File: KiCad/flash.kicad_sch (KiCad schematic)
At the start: 3 parts, among them IC4 W25Q32JWSNIQ

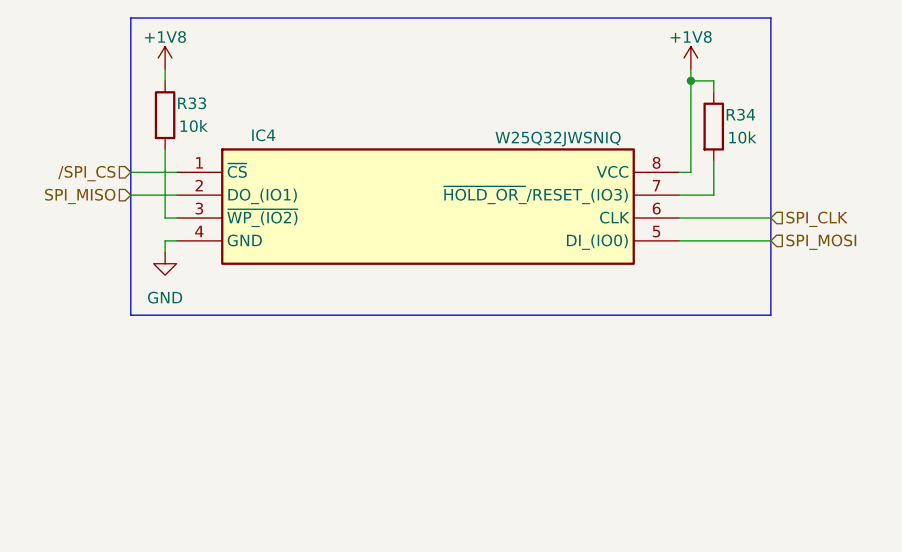
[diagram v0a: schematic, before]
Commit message: Added some TODOs, fixed some TODOs
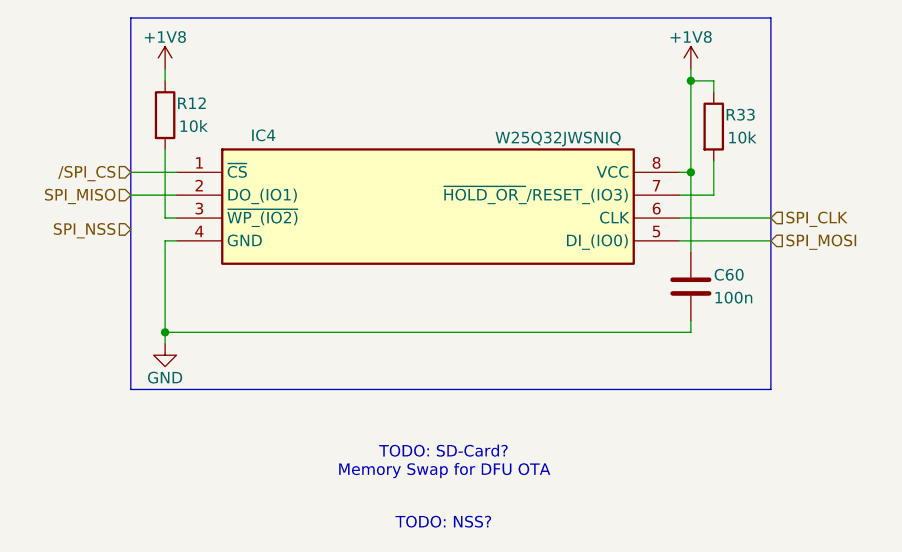
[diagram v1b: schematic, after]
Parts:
- added C60: 100n, Capacitor_SMD:C_0402_1005Metric, symbol Device:C
- renumbered R33 to R12, R34 to R33
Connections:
- net +1V8: now also C60.1
- net GND: now also C60.2
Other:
- note added: "TODO: NSS?"
- note added: "TODO: SD-Card? Memory Swap for DFU OTA"
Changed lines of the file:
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@@
 	(rectangle
 		(start 132.08 37.465)
-		(end 203.2 70.485)
+		(end 203.2 78.74)
 		(stroke
 			(width 0)
@@
 		(fill
 			(type none)
+		)
+	)
+	(text "TODO: NSS?"
+		(exclude_from_sim no)
+		(at 166.878 93.726 0)
+		(effects
+			(font
+				(size 1.27 1.27)
+			)
+		)
+	)
+	(text "TODO: SD-Card?\nMemory Swap for DFU OTA"
+		(exclude_from_sim no)
+		(at 166.878 86.868 0)
+		(effects
+			(font
+				(size 1.27 1.27)
+			)
 		)
 	)
@@
 		(color 0 0 0 0)
 	)
+	(junction
+		(at 135.89 72.39)
+		(diameter 0)
+		(color 0 0 0 0)
+	)
+	(junction
+		(at 194.31 54.61)
+		(diameter 0)
+		(color 0 0 0 0)
+	)
 	(wire
 		(pts
@@
 	(wire
 		(pts
+			(xy 135.89 73.66) (xy 135.89 72.39)
+		)
+		(stroke
+			(width 0)
+			(type default)
+		)
+	)
+	(wire
+		(pts
 			(xy 196.85 44.45) (xy 194.31 44.45)
 		)
@@
 	(wire
 		(pts
-			(xy 135.89 62.23) (xy 135.89 63.5)
-		)
-		(stroke
-			(width 0)
-			(type default)
-		)
-	)
-	(wire
-		(pts
 			(xy 135.89 43.18) (xy 135.89 44.45)
 		)
@@
 	(wire
 		(pts
+			(xy 194.31 72.39) (xy 194.31 71.12)
+		)
+		(stroke
+			(width 0)
+			(type default)
+		)
+	)
+	(wire
+		(pts
+			(xy 135.89 72.39) (xy 194.31 72.39)
+		)
+		(stroke
+			(width 0)
+			(type default)
+		)
+	)
+	(wire
+		(pts
 			(xy 137.16 59.69) (xy 135.89 59.69)
 		)
@@
 		(pts
 			(xy 132.08 54.61) (xy 137.16 54.61)
+		)
+		(stroke
+			(width 0)
+			(type default)
+		)
+	)
+	(wire
+		(pts
+			(xy 135.89 62.23) (xy 135.89 72.39)
+		)
+		(stroke
+			(width 0)
+			(type default)
+		)
+	)
+	(wire
+		(pts
+			(xy 194.31 54.61) (xy 194.31 63.5)
 		)
 		(stroke
@@
 		)
 	)
+	(hierarchical_label "SPI_NSS"
+		(shape input)
+		(at 132.08 60.96 180)
+		(effects
+			(font
+				(size 1.27 1.27)
+			)
+			(justify right)
+		)
+	)
 	(hierarchical_label "SPI_MOSI"
 		(shape input)
@@
 	(symbol
 		(lib_id "power:GND")
-		(at 135.89 63.5 0)
+		(at 135.89 73.66 0)
 		(unit 1)
 		(exclude_from_sim no)
@@
 		(on_board yes)
 		(dnp no)
-		(fields_autoplaced yes)
-		(property "Reference" "#PWR050"
-			(at 135.89 69.85 0)
+		(property "Reference" "#PWR048"
+			(at 135.89 80.01 0)
 			(effects
 				(font
@@
 		)
 		(property "Value" "GND"
-			(at 135.89 68.58 0)
+			(at 135.89 77.47 0)
 			(effects
 				(font
@@
 		)
 		(property "Footprint" ""
-			(at 135.89 63.5 0)
+			(at 135.89 73.66 0)
 			(effects
 				(font
@@
 		)
 		(property "Datasheet" ""
-			(at 135.89 63.5 0)
+			(at 135.89 73.66 0)
 			(effects
 				(font
@@
 		)
 		(property "Description" "Power symbol creates a global label with name \"GND\" , ground"
-			(at 135.89 63.5 0)
+			(at 135.89 73.66 0)
 			(effects
 				(font
@@
 		)
 		(instances
-			(project ""
-				(path "/643c756f-a801-466b-9148-7370ee6a5e00/75654986-1960-401a-97fe-a40bfa802dfa"
-					(reference "#PWR050")
+			(project "STDC"
+				(path "/643c756f-a801-466b-9148-7370ee6a5e00/a5768ca1-322e-4c77-bc87-c3070b355a8f"
+					(reference "#PWR048")
 					(unit 1)
 				)
@@
 		(on_board yes)
 		(dnp no)
-		(property "Reference" "#PWR049"
+		(property "Reference" "#PWR021"
 			(at 194.31 46.99 0)
 			(effects
@@
 		)
 		(instances
-			(project ""
-				(path "/643c756f-a801-466b-9148-7370ee6a5e00/75654986-1960-401a-97fe-a40bfa802dfa"
-					(reference "#PWR049")
+			(project "STDC"
+				(path "/643c756f-a801-466b-9148-7370ee6a5e00/a5768ca1-322e-4c77-bc87-c3070b355a8f"
+					(reference "#PWR021")
 					(unit 1)
 				)
@@
 		(on_board yes)
 		(dnp no)
-		(property "Reference" "R34"
+		(property "Reference" "R33"
 			(at 198.12 48.26 0)
 			(effects
@@
 		(instances
 			(project "STDC"
-				(path "/643c756f-a801-466b-9148-7370ee6a5e00/75654986-1960-401a-97fe-a40bfa802dfa"
-					(reference "R34")
+				(path "/643c756f-a801-466b-9148-7370ee6a5e00/a5768ca1-322e-4c77-bc87-c3070b355a8f"
+					(reference "R33")
 					(unit 1)
 				)
@@
 		(on_board yes)
 		(dnp no)
-		(property "Reference" "R33"
+		(property "Reference" "R12"
 			(at 137.16 46.99 0)
 			(effects
@@
 		)
 		(instances
-			(project ""
-				(path "/643c756f-a801-466b-9148-7370ee6a5e00/75654986-1960-401a-97fe-a40bfa802dfa"
-					(reference "R33")
+			(project "STDC"
+				(path "/643c756f-a801-466b-9148-7370ee6a5e00/a5768ca1-322e-4c77-bc87-c3070b355a8f"
+					(reference "R12")
+					(unit 1)
+				)
+			)
+		)
+	)
+	(symbol
+		(lib_id "Device:C")
+		(at 194.31 67.31 0)
+		(unit 1)
+		(exclude_from_sim no)
+		(in_bom yes)
+		(on_board yes)
+		(dnp no)
+		(property "Reference" "C60"
+			(at 196.85 66.04 0)
+			(effects
+				(font
+					(size 1.27 1.27)
+				)
+				(justify left)
+			)
+		)
+		(property "Value" "100n"
+			(at 196.85 68.58 0)
+			(effects
+				(font
+					(size 1.27 1.27)
+				)
+				(justify left)
+			)
+		)
+		(property "Footprint" "Capacitor_SMD:C_0402_1005Metric"
+			(at 195.2752 71.12 0)
+			(effects
+				(font
+					(size 1.27 1.27)
+				)
+				(hide yes)
+			)
+		)
+		(property "Datasheet" "~"
+			(at 194.31 67.31 0)
+			(effects
+				(font
+					(size 1.27 1.27)
+				)
+				(hide yes)
+			)
+		)
+		(property "Description" "Unpolarized capacitor"
+			(at 194.31 67.31 0)
+			(effects
+				(font
+					(size 1.27 1.27)
+				)
+				(hide yes)
+			)
+		)
+		(pin "2"
+		)
+		(pin "1"
+		)
+		(instances
+			(project "STDC"
+				(path "/643c756f-a801-466b-9148-7370ee6a5e00/a5768ca1-322e-4c77-bc87-c3070b355a8f"
+					(reference "C60")
 					(unit 1)
 				)
@@
 		)
 		(instances
-			(project ""
-				(path "/643c756f-a801-466b-9148-7370ee6a5e00/75654986-1960-401a-97fe-a40bfa802dfa"
+			(project "STDC"
+				(path "/643c756f-a801-466b-9148-7370ee6a5e00/a5768ca1-322e-4c77-bc87-c3070b355a8f"
 					(reference "IC4")
 					(unit 1)
@@
 		(on_board yes)
 		(dnp no)
-		(property "Reference" "#PWR048"
+		(property "Reference" "#PWR016"
 			(at 135.89 46.99 0)
 			(effects
@@
 		(instances
 			(project "STDC"
-				(path "/643c756f-a801-466b-9148-7370ee6a5e00/75654986-1960-401a-97fe-a40bfa802dfa"
-					(reference "#PWR048")
+				(path "/643c756f-a801-466b-9148-7370ee6a5e00/a5768ca1-322e-4c77-bc87-c3070b355a8f"
+					(reference "#PWR016")
 					(unit 1)
 				)
